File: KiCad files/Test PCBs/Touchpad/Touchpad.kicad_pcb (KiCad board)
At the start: 2 copper layers, 100 x 51.2 mm, 63 parts, among them J1 Conn_01x08_Male, J2 Conn_01x03_Male, U1 TTP223-BA6, U2 TTP223-BA6, U3 TTP223-BA6, U4 TTP223-BA6, U5 TTP223-BA6, U6 TTP223-BA6

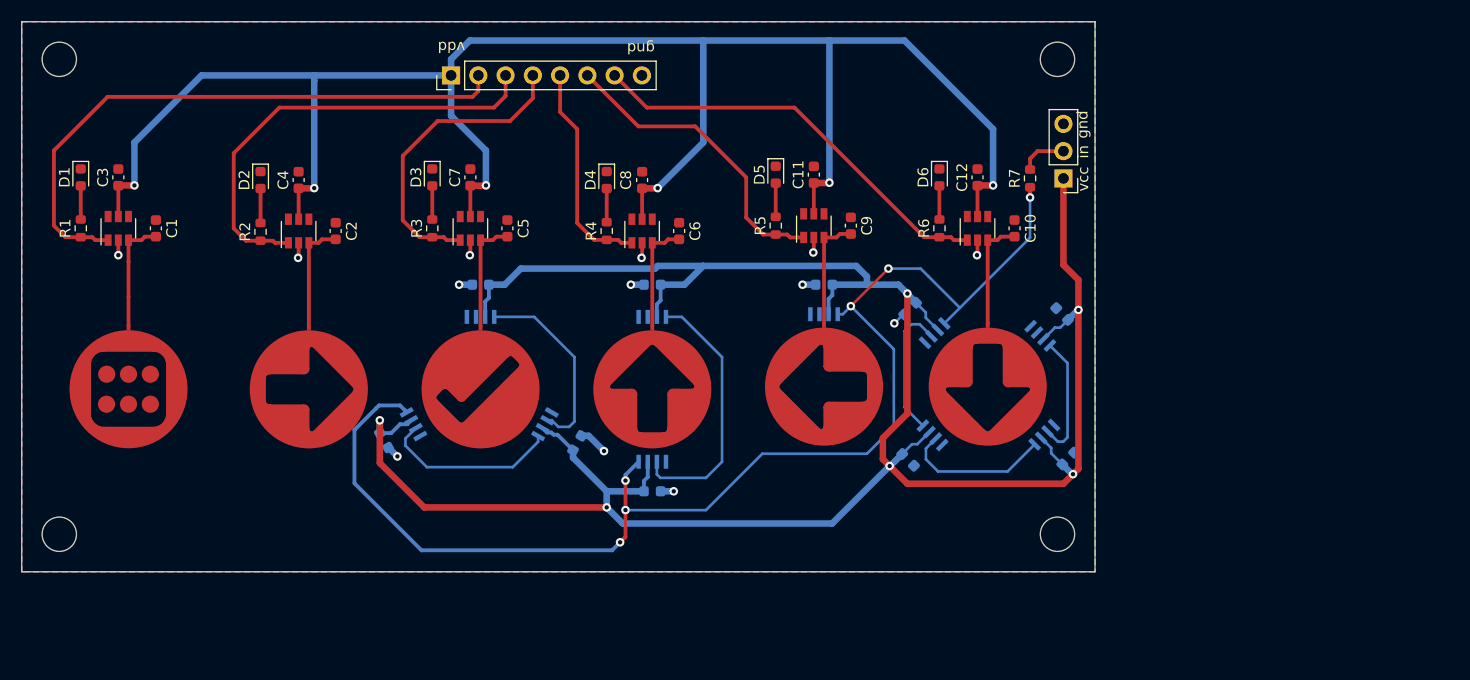
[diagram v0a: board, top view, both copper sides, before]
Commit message: update
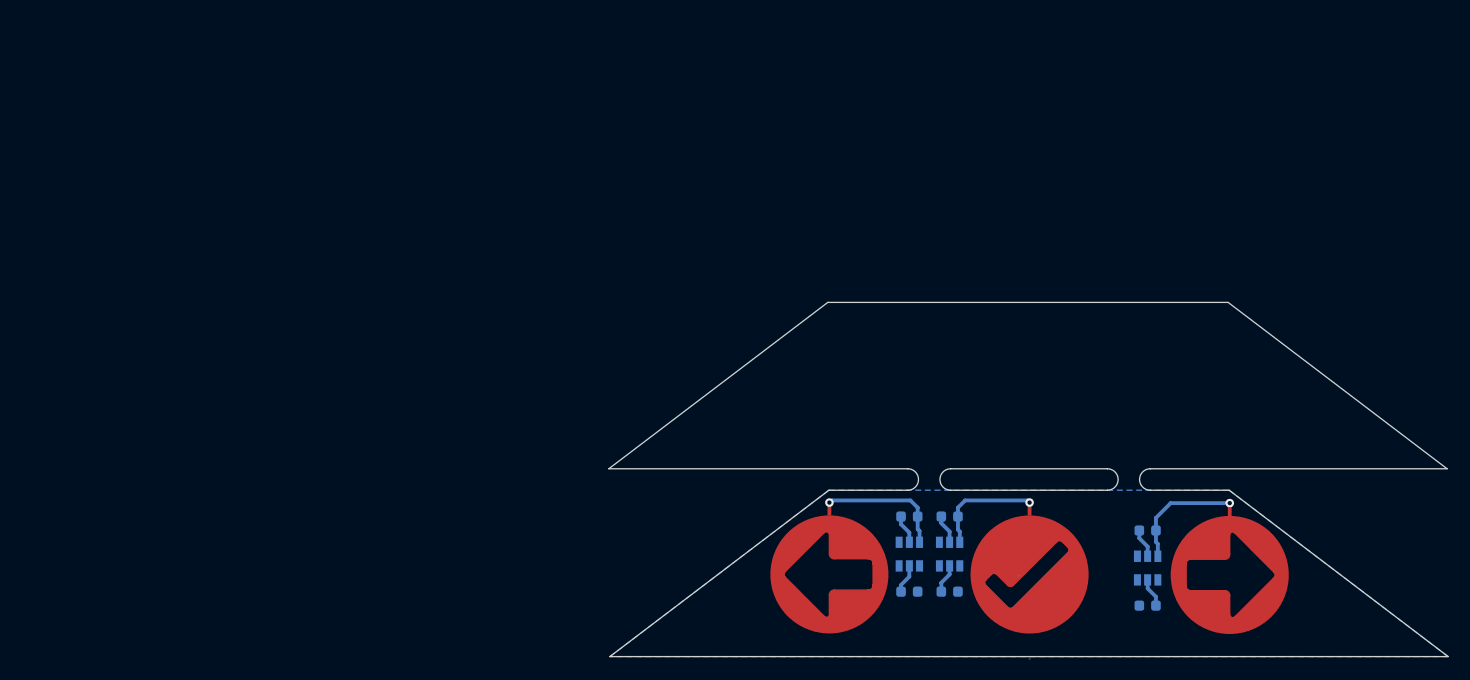
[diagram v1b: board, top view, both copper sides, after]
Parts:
- removed C1, C10, C6: 0-50 pF, Capacitor_SMD:C_0603_1608Metric
- removed C12, C13, C14, C15, C16, C17, C18, C19, C20, C21, C22, C3, C8: 100n, Capacitor_SMD:C_0603_1608Metric
- removed D1, D2, D3, D4, D5, D6: LED_Small, LED_SMD:LED_0603_1608Metric
- removed D10, D11, D12, D13, D14, D15, D16, D7, D8, D9: WS2812-4020, Touchpad:WS2812-4020
- removed H1, H2, H3, H4: MountingHole, MountingHole:MountingHole_3.2mm_M3
- removed J1: Conn_01x08_Male, Connector_PinHeader_2.54mm:PinHeader_1x08_P2.54mm_Vertical
- removed J2: Conn_01x03_Male, Connector_PinHeader_2.54mm:PinHeader_1x03_P2.54mm_Vertical
- removed R1, R2, R3, R4, R5, R6, R7: 470, Resistor_SMD:R_0603_1608Metric
- removed TP1: TestPoint, Touchpad:TP_11mm_kocka
- removed TP5: TestPoint, Touchpad:TP_11mm_strelicaGore
- removed TP6: TestPoint, Touchpad:TP_11mm_strelicaDolje
- removed U1, U4, U6: TTP223-BA6, Package_TO_SOT_SMD:SOT-23-6
- C11, C2, C4, C5, C7, C9, U2, U3, U5: moved to B.Cu
- moved C4 88.5 mm to (209.9, 109.4), turned to 180 degrees
- moved TP4 87.5 mm to (217.6, 106.5)
- moved U2 85.1 mm to (209.9, 105.9), turned to -90 degrees
- moved C2 80.6 mm to (209.9, 102.4), turned to 180 degrees
- moved C7 59.0 mm to (191.4, 108.1), turned to 0 degrees
- moved U3 54.0 mm to (191.4, 104.6), turned to -90 degrees
- moved TP2 54.0 mm to (198.9, 106.5)
- moved C5 49.2 mm to (191.4, 101.1), turned to 180 degrees
- moved C11 39.9 mm to (187.7, 108.1), turned to 0 degrees
- moved U5 31.9 mm to (187.7, 104.6), turned to -90 degrees
- moved C9 27.6 mm to (187.7, 101.1), turned to 180 degrees
- moved TP3 17.5 mm to (180.2, 106.5)
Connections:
- U2 pad 4: Net-(U2-Pad4) -> unconnected-(U2-Pad4)
- U2 pad 6: Net-(U2-Pad6) -> unconnected-(U2-Pad6)
- U3 pad 4: Net-(U3-Pad4) -> unconnected-(U3-Pad4)
- U3 pad 6: Net-(U3-Pad6) -> unconnected-(U3-Pad6)
- U5 pad 4: Net-(U5-Pad4) -> unconnected-(U5-Pad4)
- U5 pad 6: Net-(U5-Pad6) -> unconnected-(U5-Pad6)
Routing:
- net VCC: track 218.0 -> 0.00 mm, vias 6 -> 0
- net +5V: track 174.4 -> 8.16 mm, vias 6 -> 0
- net Net-(D11-Pad1): track 118.7 -> 0.00 mm, vias 6 -> 0
- net TP1: track 55.9 -> 0.00 mm
- net TP2: track 42.1 -> 0.00 mm
- net TP6: track 39.2 -> 0.00 mm
- net TP5: track 28.6 -> 0.00 mm
- net TP3: track 28.6 -> 0.00 mm
- net Net-(D14-Pad3): track 24.5 -> 0.00 mm
- net TP4: track 20.3 -> 0.00 mm
- net Net-(D12-Pad3): track 18.0 -> 0.00 mm
- net Net-(D11-Pad3): track 16.7 -> 0.00 mm
- net Net-(D8-Pad3): track 14.0 -> 0.00 mm
- net Net-(D7-Pad3): track 12.8 -> 0.00 mm
- net Net-(D10-Pad1): track 11.7 -> 0.00 mm
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- removed copper zone on F.Cu, net GND
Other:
- board size 100 x 51.2 mm -> 78.2 x 33.2 mm
- board text removed: "gnd"
- board text removed: "in"
- board text removed: "vcc"
- board text removed: "vdd"
